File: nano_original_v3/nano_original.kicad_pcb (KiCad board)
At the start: 2 copper layers, 43.2 x 17.8 mm, 29 parts, among them J1 USB_B_Micro, J2 Conn_01x15, J3 Conn_01x15, J4 Conn_02x03_Odd_Even, SW1 SW_Push, U1 LM1117MP-5.0, U2 FT231XS, U3 ATmega328P-M, Y1 16MHz

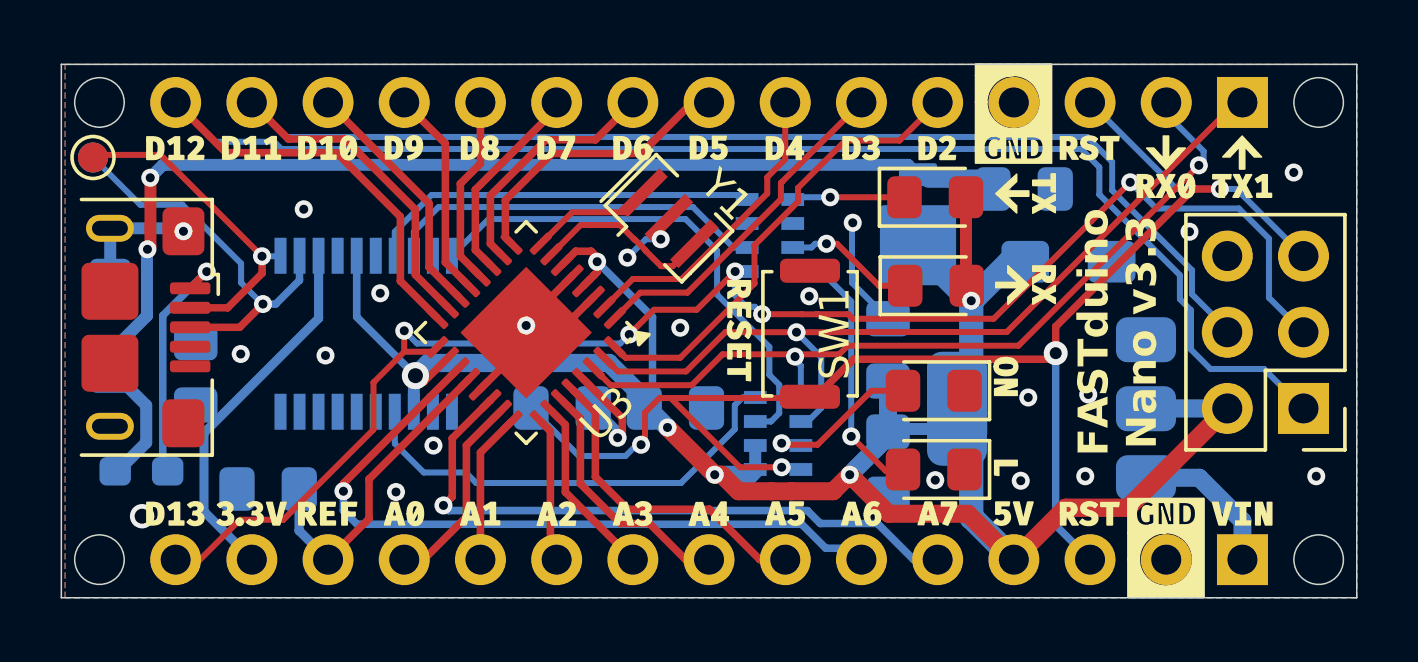
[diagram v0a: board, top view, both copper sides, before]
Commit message: updated BOM
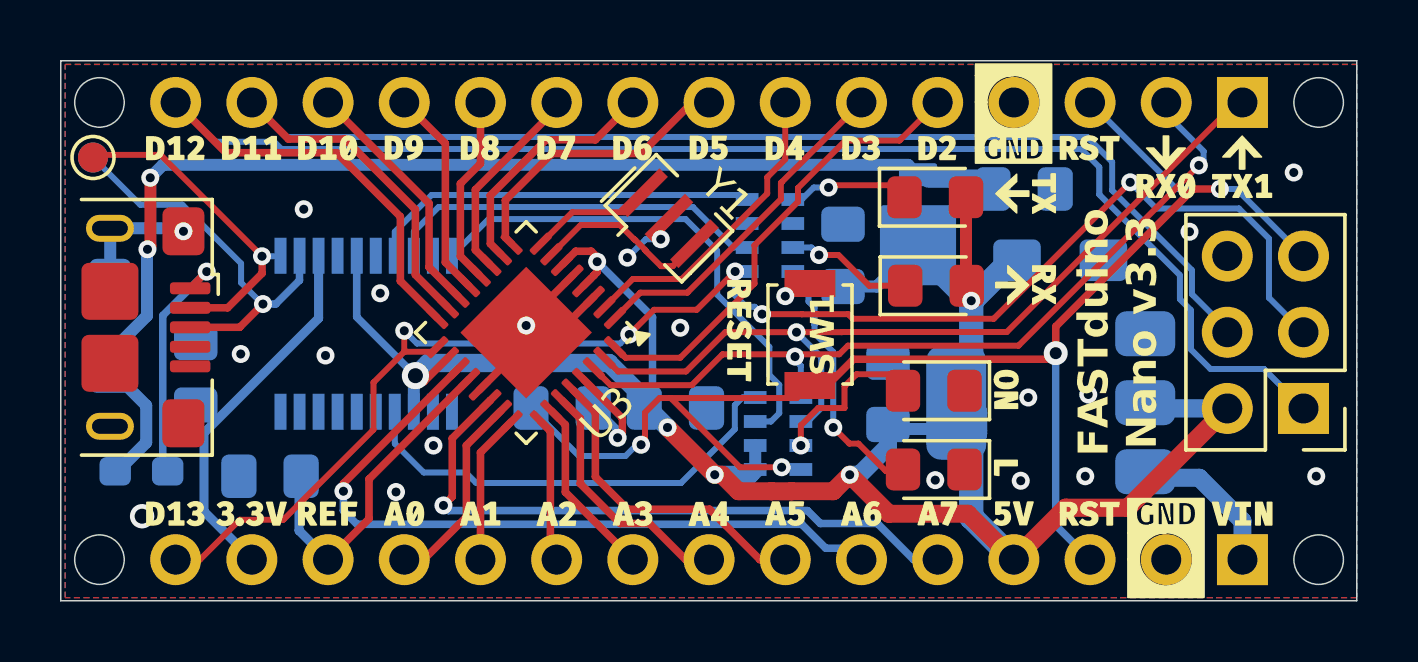
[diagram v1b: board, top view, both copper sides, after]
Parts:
- J2, J3: footprint Connector_PinSocket_2.54mm:PinSocket_1x15_P2.54mm_Vertical -> Connector_PinHeader_2.54mm:PinHeader_1x15_P2.54mm_Vertical; moved to B.Cu
- SW1: footprint Button_Switch_SMD:SW_Push_SPST_NO_Alps_SKRK -> Button_Switch_SMD:SW_SPST_B3U-1000P
- Silkscreen_Front: footprint NanoV3.3:Silkscreen_Front -> silk:Silkscreen_Front
- U3: value ATmega328P-M -> ATmega328P-MUR
- moved C4 3.49 mm to (85.2, 80.5)
- moved C1 2.32 mm to (86.7, 85.1), turned to 90 degrees
- moved C8 0.43 mm to (66.1, 87.8)
- moved C3 0.28 mm to (92.5, 80.7)
- moved U1 0.20 mm to (92.2, 85.4)
- turned J2 to 90 degrees
- turned J3 to 90 degrees
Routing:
- net GND: track 17.3 -> 13.6 mm, vias 21 -> 20
- net +5V: track 79.5 -> 80.9 mm
- net /AREF: track 10.7 -> 11.6 mm
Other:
- board size 43.2 x 17.8 mm -> 43.2 x 18 mm
